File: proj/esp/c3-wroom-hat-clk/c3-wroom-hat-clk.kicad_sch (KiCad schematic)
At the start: 13 parts, among them J1 OUT1, J2 OUT2, U1 LTC-4627JG, U2 74HC595, U3 74HC595

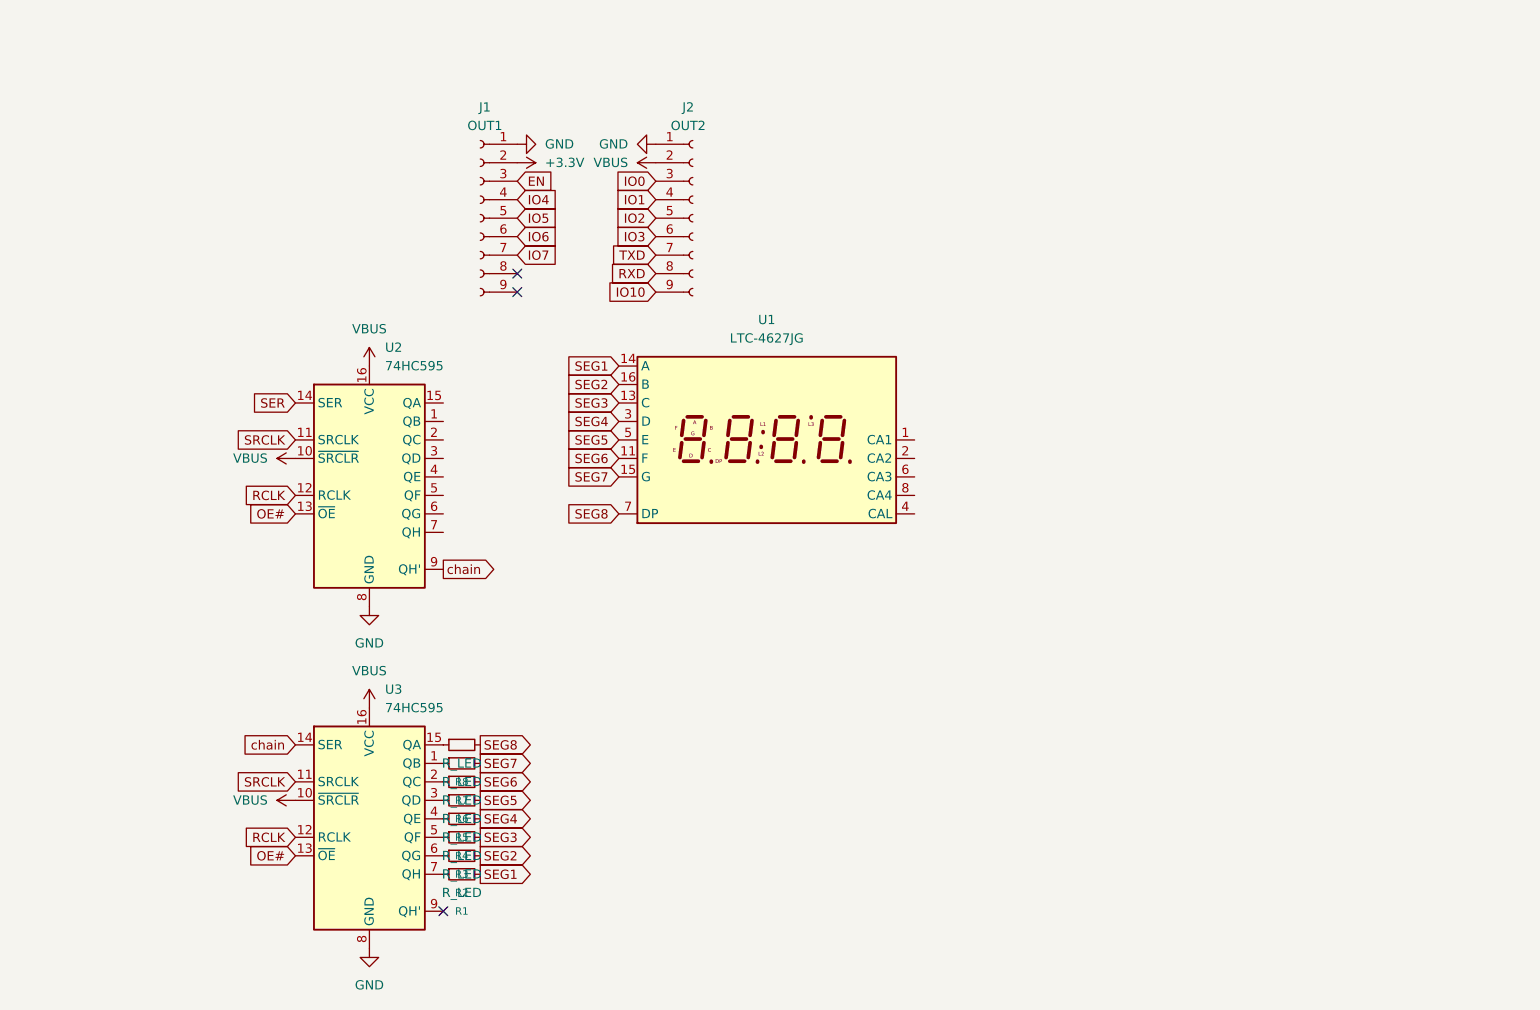
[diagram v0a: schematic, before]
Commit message: -
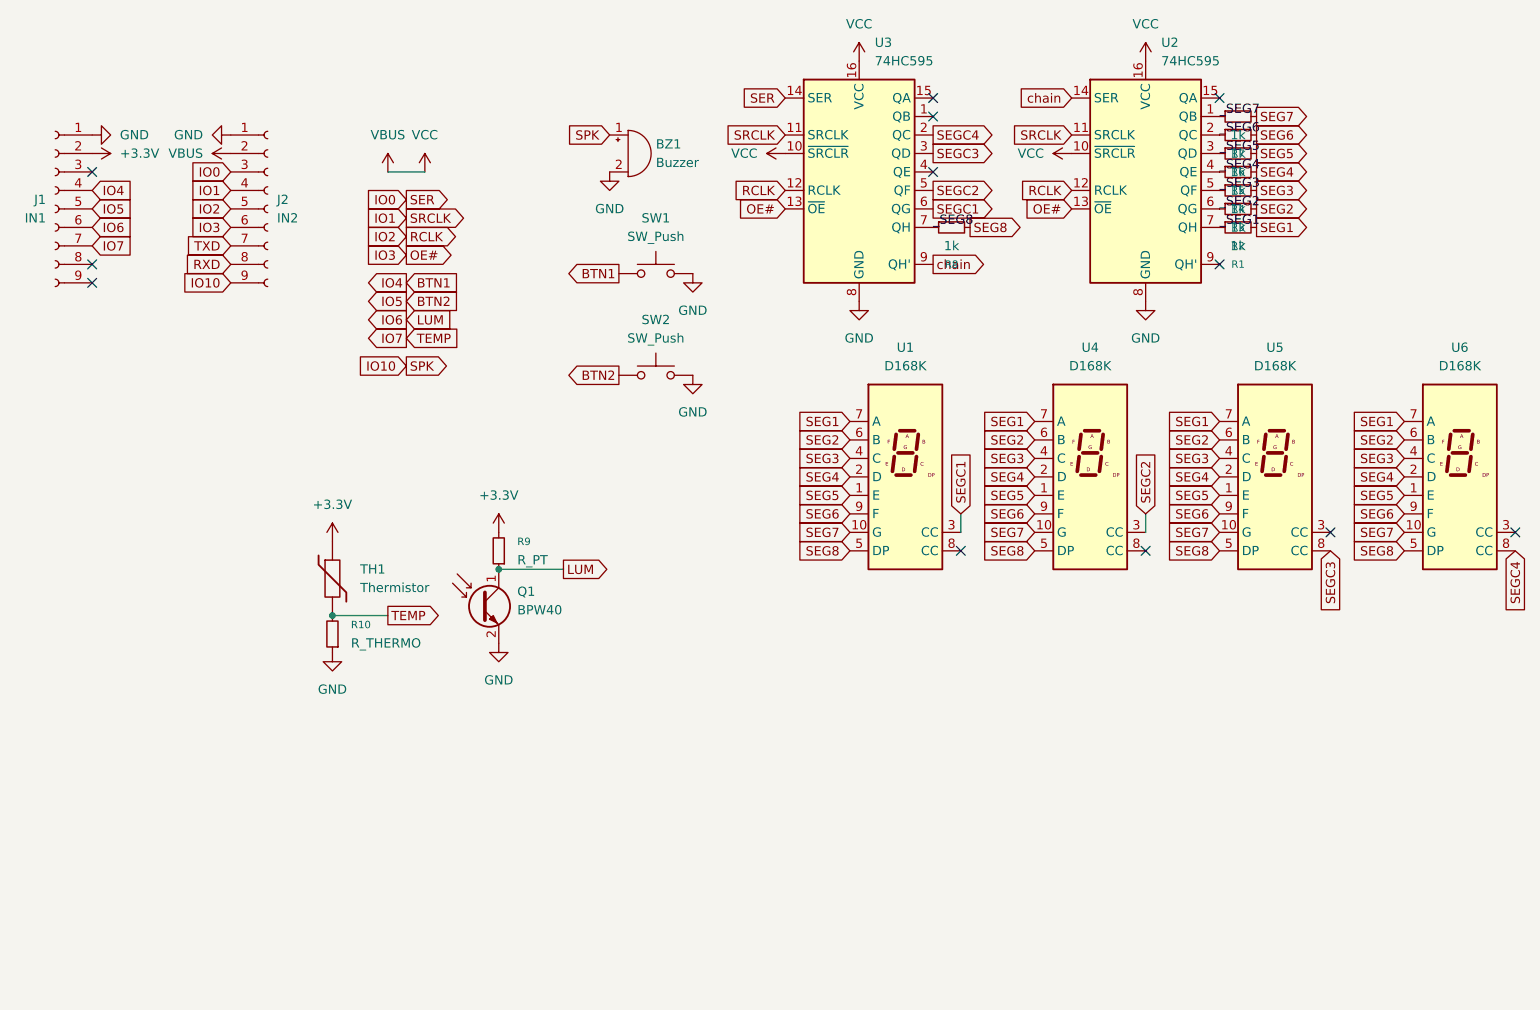
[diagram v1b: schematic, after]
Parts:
- removed U1: LTC-4627JG, Display_7Segment:LTC-4627Jx, symbol Display_Character:LTC-4627JG
- added BZ1: Buzzer, Buzzer_Beeper:Buzzer_TDK_PS1240P02BT_D12.2mm_H6.5mm, symbol Device:Buzzer
- added Q1: BPW40, LED_THT:LED_D5.0mm_Clear, symbol Sensor_Optical:BPW40
- added R10: R_THERMO, Resistor_SMD:R_0603_1608Metric, symbol Device:R_Small
- added R9: R_PT, Resistor_SMD:R_0603_1608Metric, symbol Device:R_Small
- added SW1, SW2: SW_Push, Library:alps-skrg, symbol Switch:SW_Push
- added TH1: Thermistor, Resistor_SMD:R_0603_1608Metric, symbol Device:Thermistor
- added U1, U4, U5, U6: D168K, Display_7Segment:D1X8K, symbol Display_Character:D168K
- J1: value OUT1 -> IN1
- J2: value OUT2 -> IN2
- R1, R2, R3, R4, R5, R6, R7, R8: value R_LED -> 1k; footprint (none) -> Resistor_SMD:R_0603_1608Metric
- U2, U3: footprint (none) -> Package_SO:TSSOP-16_4.4x5mm_P0.65mm
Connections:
- net OE# is gone; now on net IO3: U2.13 (~{OE}), U3.13 (~{OE})
- net RCLK is gone; now on net IO2: U2.12 (RCLK), U3.12 (RCLK)
- net SER is gone; now on net chain: U2.14 (SER)
- net SRCLK is gone; now on net IO1: U2.11 (SRCLK), U3.11 (SRCLK)
- net +3.3V: now also R9.2, TH1.1
- net GND: now also BZ1.2 (-), Q1.2 (E), R10.1, SW1.2, SW2.2
- net IO0: now also U3.14 (SER)
- net IO10: now also BZ1.1 (+)
- net IO6: now also Q1.1 (C), R9.1
- net IO7: now also R10.2, TH1.2
- net SEG1: now also U1.7 (A), U4.7 (A), U5.7 (A), U6.7 (A)
- net SEG2: now also U1.6 (B), U4.6 (B), U5.6 (B), U6.6 (B)
- net SEG3: now also U1.4 (C), U4.4 (C), U5.4 (C), U6.4 (C)
- net SEG4: now also U1.2 (D), U4.2 (D), U5.2 (D), U6.2 (D)
- net SEG5: now also U1.1 (E), U4.1 (E), U5.1 (E), U6.1 (E)
- net SEG6: now also U1.9 (F), U4.9 (F), U5.9 (F), U6.9 (F)
- net SEG7: now also U1.10 (G), U4.10 (G), U5.10 (G), U6.10 (G)
- net SEG8: now also U1.5 (DP), U4.5 (DP), U5.5 (DP), U6.5 (DP)
- net chain: now also U3.9 (QH'); no longer U2.9 (QH'), U3.14 (SER)
- net SEGC4: now reaches U3.2 (QC)
- net SEGC4: now also U6.8 (CC); no longer R6.1
- net SEGC2: now reaches U3.5 (QF)
- net SEGC2: now also U4.3 (CC); no longer R3.1
- net SEGC1: now reaches U3.6 (QG)
- net SEGC1: now also U1.3 (CC); no longer R2.1
- net _SEG1: now reaches R1.1
- net _SEG1: now also U2.7 (QH); no longer U3.7 (QH)
- net SEGC3: now reaches U3.3 (QD)
- net SEGC3: now also U5.8 (CC); no longer R5.1
- net at U3.1 (QB): no longer R7.1
- net at U3.15 (QA): no longer R8.1
- net at U3.4 (QE): no longer R4.1
- net _SEG7: now reaches U2.1 (QB)
- net _SEG7: now also R7.1
- net _SEG6: now reaches U2.2 (QC)
- net _SEG6: now also R6.1
- net _SEG5: now reaches U2.3 (QD)
- net _SEG5: now also R5.1
- net _SEG4: now reaches U2.4 (QE)
- net _SEG4: now also R4.1
- net _SEG3: now reaches U2.5 (QF)
- net _SEG3: now also R3.1
- net _SEG2: now reaches U2.6 (QG)
- net _SEG2: now also R2.1
- net EN: no longer names the net of J1.3 (Pin_3)
- net IO4 renamed BTN1
- net BTN1: now also SW1.1
- net IO5 renamed BTN2
- net BTN2: now also SW2.1
- new net _SEG8: R8.1, U3.7 (QH)
- no-connect marks 3 -> 12
